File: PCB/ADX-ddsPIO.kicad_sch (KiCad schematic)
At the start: 68 parts, among them J1 Conn_Coaxial, J2 +12V, Q1 BS170, Q2 BS170, Q3 BS170, Q5 BS170, U1 L7805, U2 74LS244, U4 CD2003GB_GP

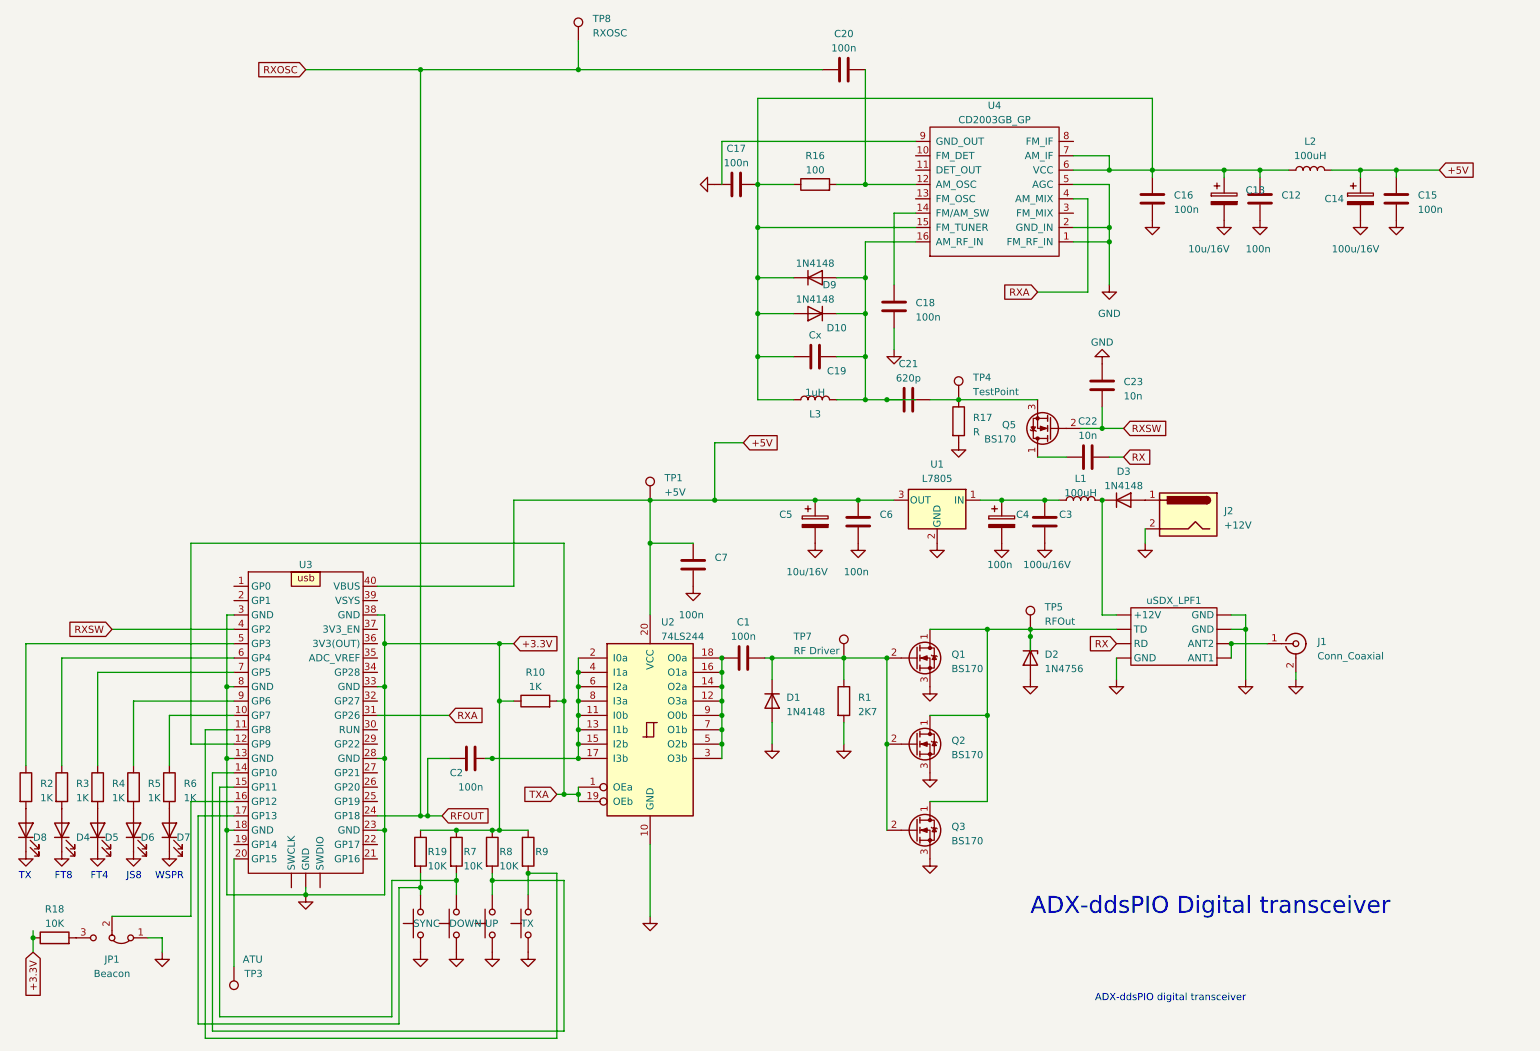
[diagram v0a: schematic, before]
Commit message: ADX-ddsPIO-V1.0
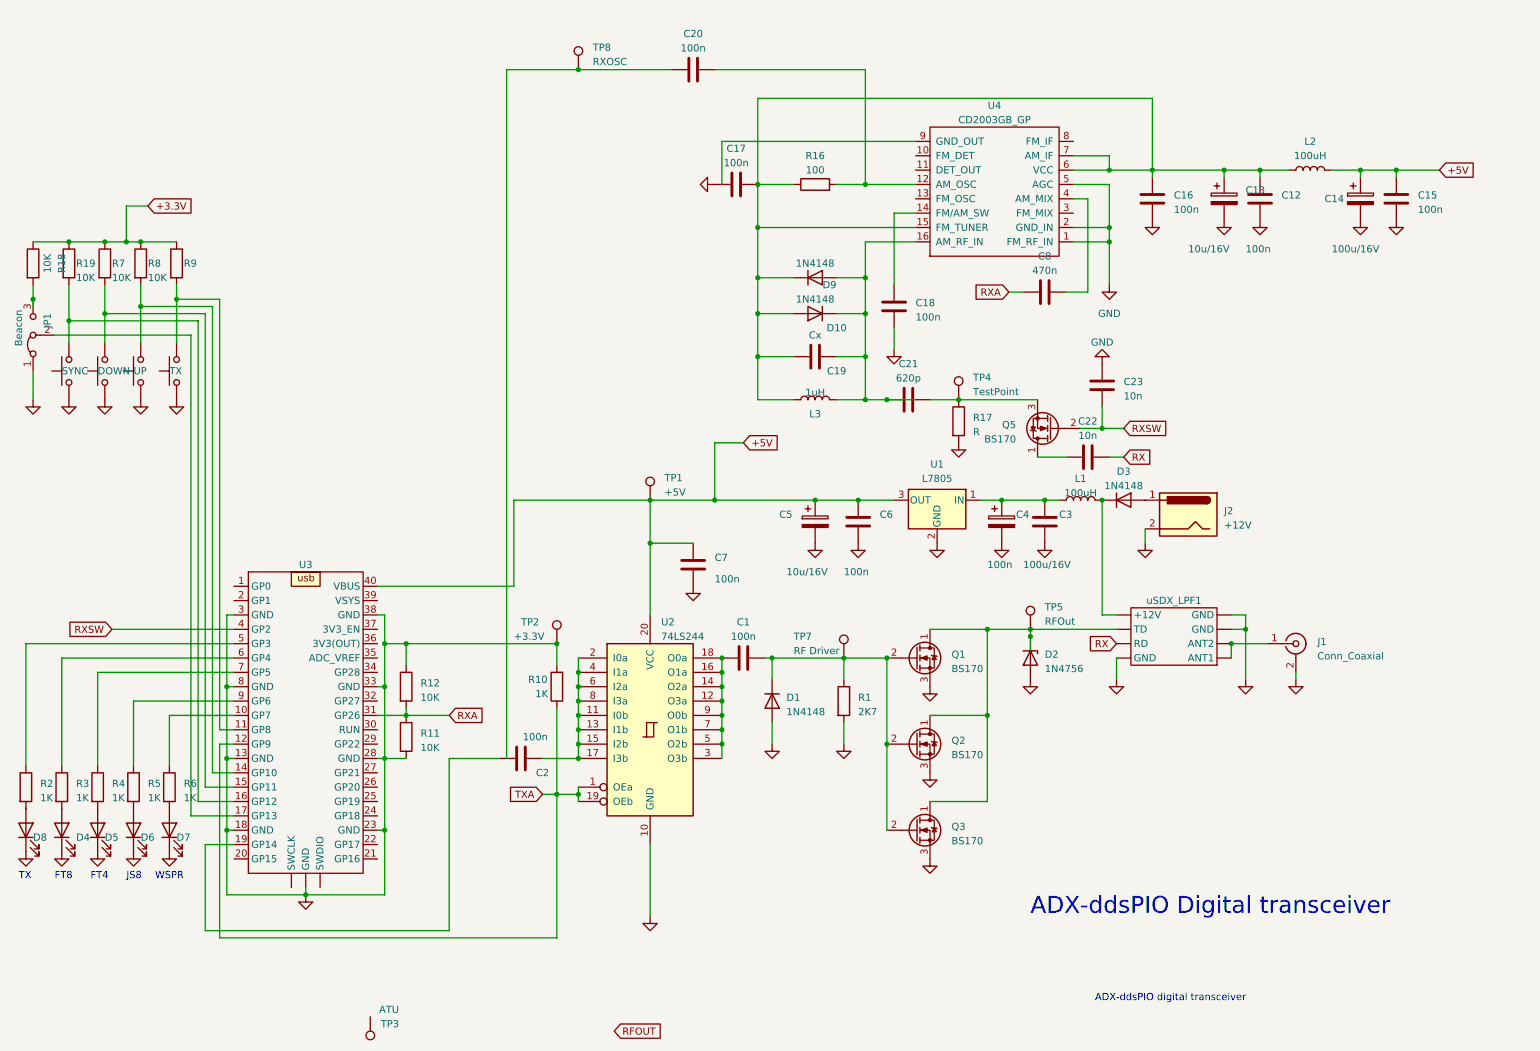
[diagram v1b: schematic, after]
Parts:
- added C8: 470n, symbol Device:C
- added R11, R12: 10K, symbol Device:R
- added TP2: +3.3V, symbol Connector:TestPoint
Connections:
- net GND: now also R10.2, R11.2, R12.1, TP2.1; no longer R10.1, R18.1, R19.1, R7.1, R8.1, R9.1
- net RFOUT: no longer C2.1, C20.1, TP8.1, U3.24 (GP18)
- net RXA: now also C8.1, R11.1, R12.2; no longer U4.4 (AM_MIX)
- net TXA: now also R10.1; no longer R10.2
- net at JP1.2 (C): now also U3.17 (GP13); no longer U3.16 (GP12)
- net at R19.2, SYNC.3 (B), SYNC.4 (B): now also U3.16 (GP12); no longer U3.17 (GP13)
- net at U3.19 (GP14): now also C2.1
- net at U3.20 (GP15): no longer TP3.1
- new net: C8.2, U4.4 (AM_MIX)
- new net: C20.1, TP8.1
- new net +3.3V: R18.1, R19.1, R7.1, R8.1, R9.1
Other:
- moved on the sheet: C2, C20, DOWN, JP1, R10, R18, R19, R7, R8, R9, SYNC, TP3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
